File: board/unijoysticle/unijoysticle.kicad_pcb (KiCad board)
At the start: 2 copper layers, 55.6 x 41.7 mm, 14 parts, among them IC1 7405, IC2 7405, J1 DB9_Female, J2 DB9_Female, J3 Barrel_Jack, SW1 SW_Push

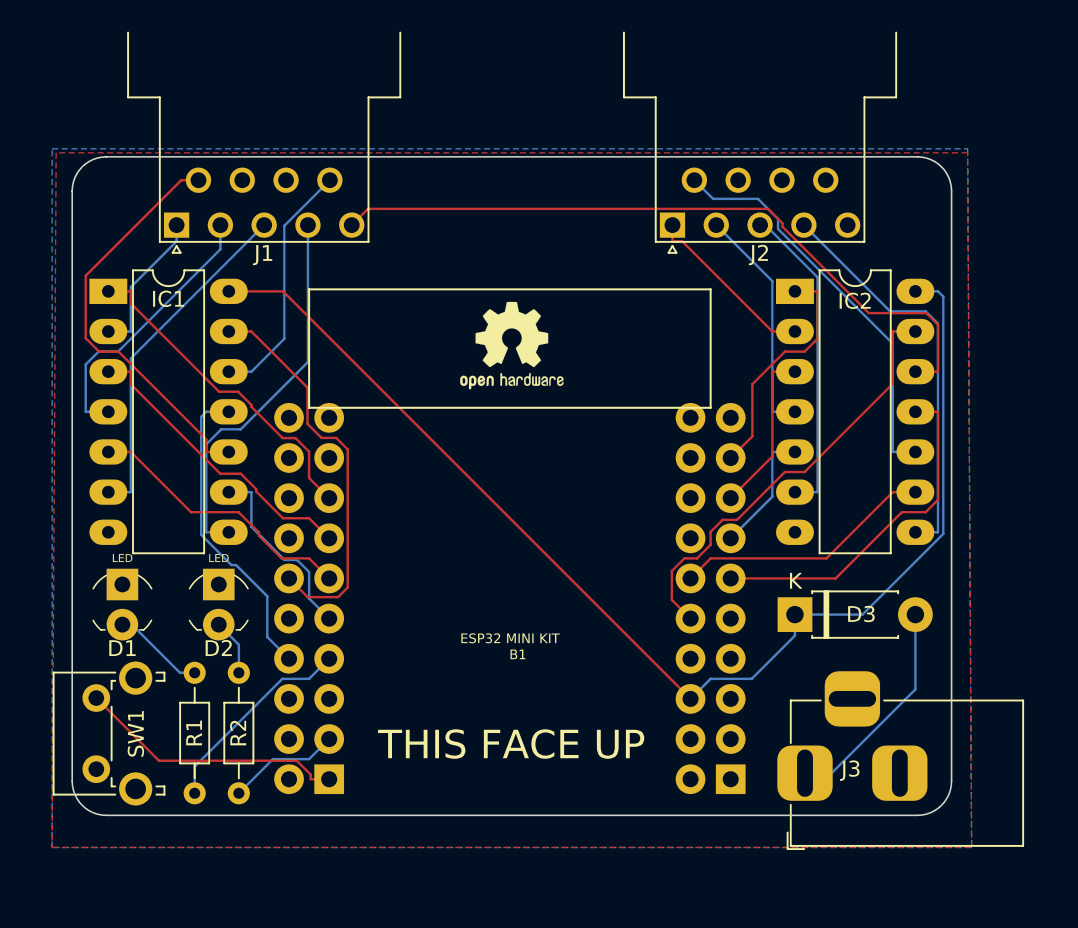
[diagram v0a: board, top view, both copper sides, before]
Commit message: layout: Rev C: Work in progress
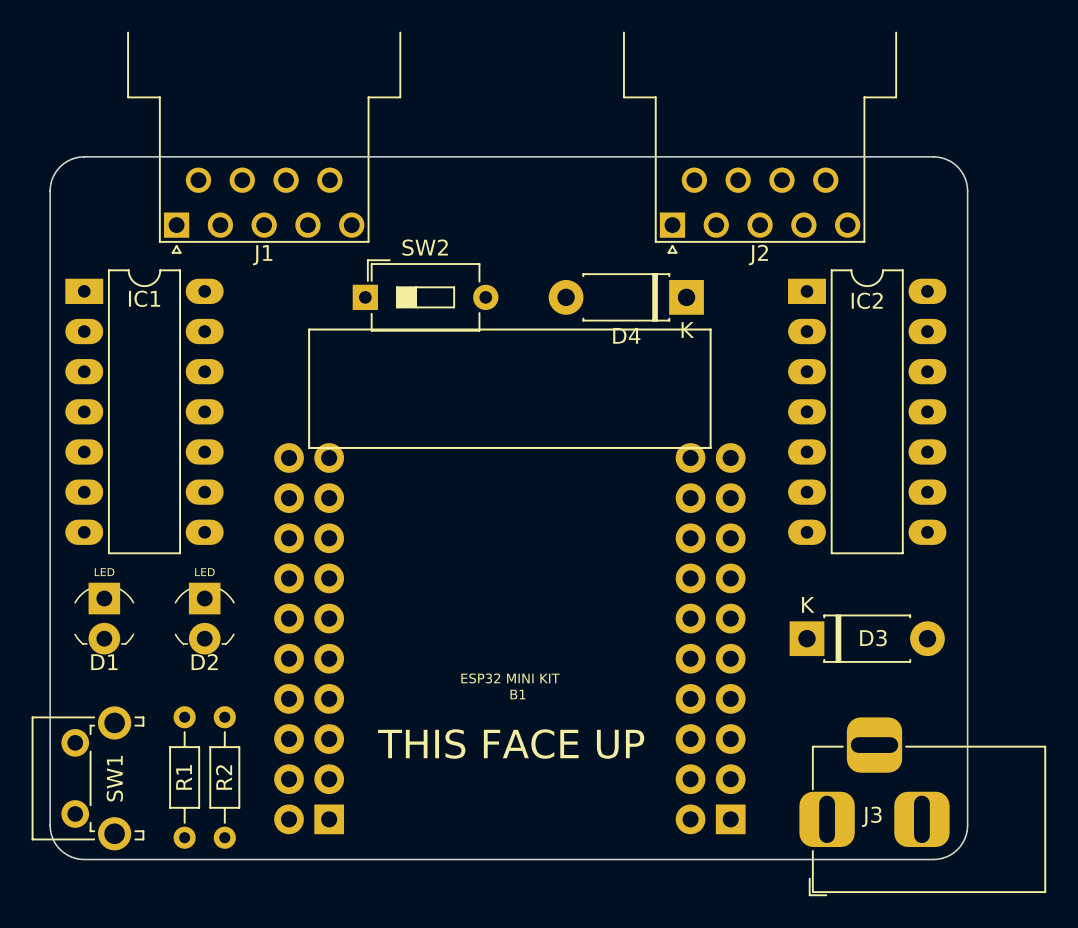
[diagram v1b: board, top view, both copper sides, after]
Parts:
- removed G***: LOGO, Parts:unijoysticle_logo
- removed REF**: OSHW-Logo2_7.3x6mm_SilkScreen, Symbol:OSHW-Logo2_7.3x6mm_SilkScreen
- added D4: 1N4001, Diode_THT:D_DO-41_SOD81_P7.62mm_Horizontal, F.Cu at (153.7, 83.8)
- added SW2: SW_SPST, Button_Switch_THT:SW_DIP_SPSTx01_Slide_6.7x4.1mm_W7.62mm_P2.54mm_LowProfile, F.Cu at (133.3, 83.8)
- R1, R2: value 100 -> 150
- moved J3 3.24 mm to (162.6, 116.8)
- moved SW1 3.13 mm to (115.0, 116.5)
- moved R2 2.95 mm to (124.5, 118.0)
- moved R1 2.88 mm to (121.9, 118.0)
- moved B1 2.54 mm to (127.3, 125.7)
- moved D3 1.70 mm to (161.3, 105.4)
- moved IC1 1.52 mm to (115.6, 83.4)
- moved D1 1.45 mm to (116.8, 105.4)
- moved D2 1.26 mm to (123.2, 105.4)
- moved IC2 0.76 mm to (161.3, 83.4)
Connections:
- IC1 pad 14: VDD -> J1POWER
- IC2 pad 14: VDD -> Net-(IC2-Pad14)
- J1 pad 7: Net-(J1-Pad7) -> J1POWER
- J2 pad 7: Net-(J2-Pad7) -> J1POWER
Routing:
- net VDD: track 77.9 -> 0.00 mm
- net J1POTY: track 45.1 -> 0.00 mm
- net GPIO_J1POTY: track 27.6 -> 0.00 mm
- net J1FIRE: track 26.1 -> 0.00 mm
- net J2RIGHT: track 25.7 -> 0.00 mm
- net J2FIRE: track 25.5 -> 0.00 mm
- net GPIO_J1POTX: track 25.1 -> 0.00 mm
- net J1RIGHT: track 24.2 -> 0.00 mm
- net GPIO_J2FIRE: track 22.2 -> 0.00 mm
- net J1LEFT: track 21.8 -> 0.00 mm
- net GPIO_J1UP: track 20.9 -> 0.00 mm
- net J2LEFT: track 20.0 -> 0.00 mm
- net GPIO_J1FIRE: track 19.7 -> 0.00 mm
- net GPIO_J1DOWN: track 18.9 -> 0.00 mm
- net J1DOWN: track 17.5 -> 0.00 mm
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- removed copper zone on B.Cu, net GND
- removed copper zone on F.Cu, net GND
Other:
- board size 55.6 x 41.7 mm -> 58 x 44.4 mm
- board text added: "Rev C"
- board text removed: "Rev B"
